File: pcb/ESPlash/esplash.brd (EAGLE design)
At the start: 100 x 70 mm, 55 parts, among them IC1 ACS712, K1 SRD-05VDC-SL-C, K2 SRD-05VDC-SL-C, K3 SRD-05VDC-SL-C, K4 SRD-05VDC-SL-C, Q1 SMD-TRANSISTORS-PNP-25V-500MA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, Q2 SMD-TRANSISTORS-PNP-25V-500MA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, Q3 SMD-TRANSISTORS-PNP-25V-500MA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, Q4 SMD-TRANSISTORS-PNP-25V-500MA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, U1 ESP-WROOM-32, U2 EL817(S)(D)(TU)-V, U3 EL817(S)(D)(TU)-V, U4 EL817(S)(D)(TU)-V, U5 EL817(S)(D)(TU)-V, Y1 ECS-.327-12.5-13X

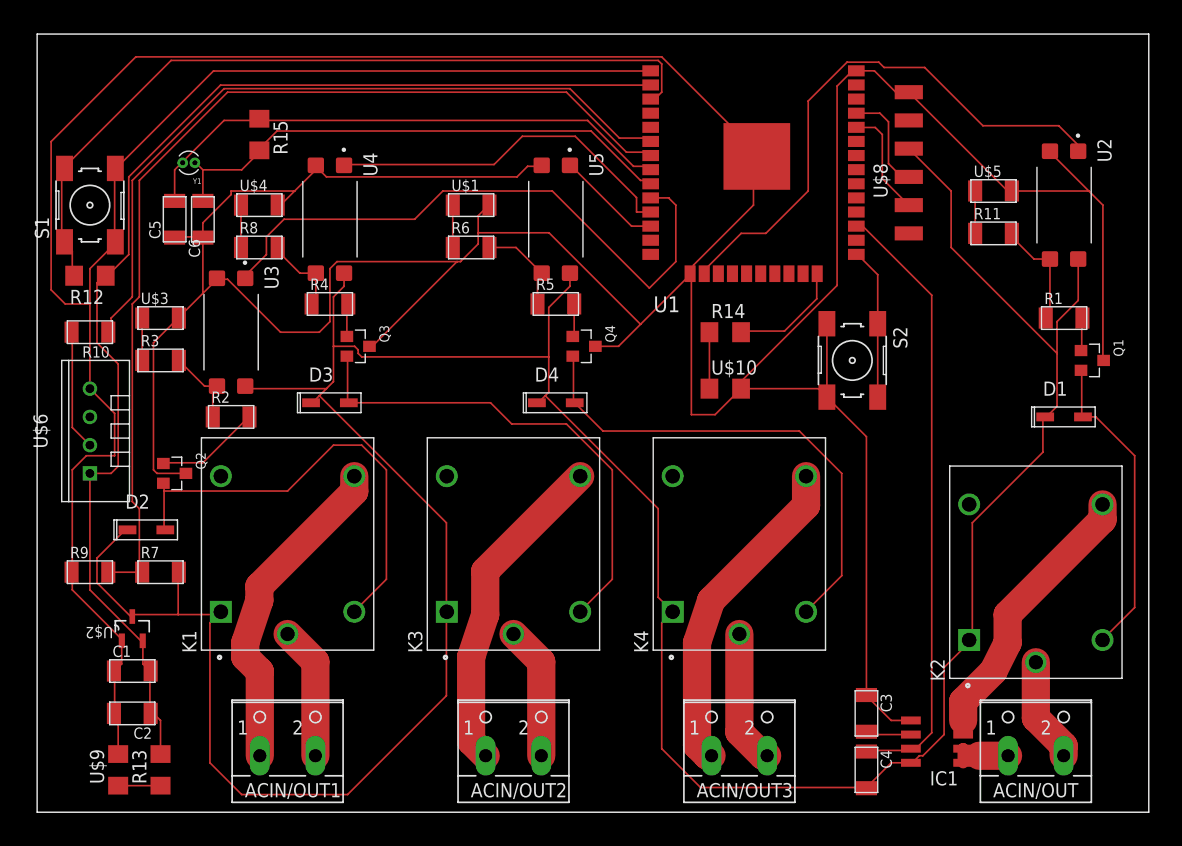
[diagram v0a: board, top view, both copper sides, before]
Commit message: pcb updates
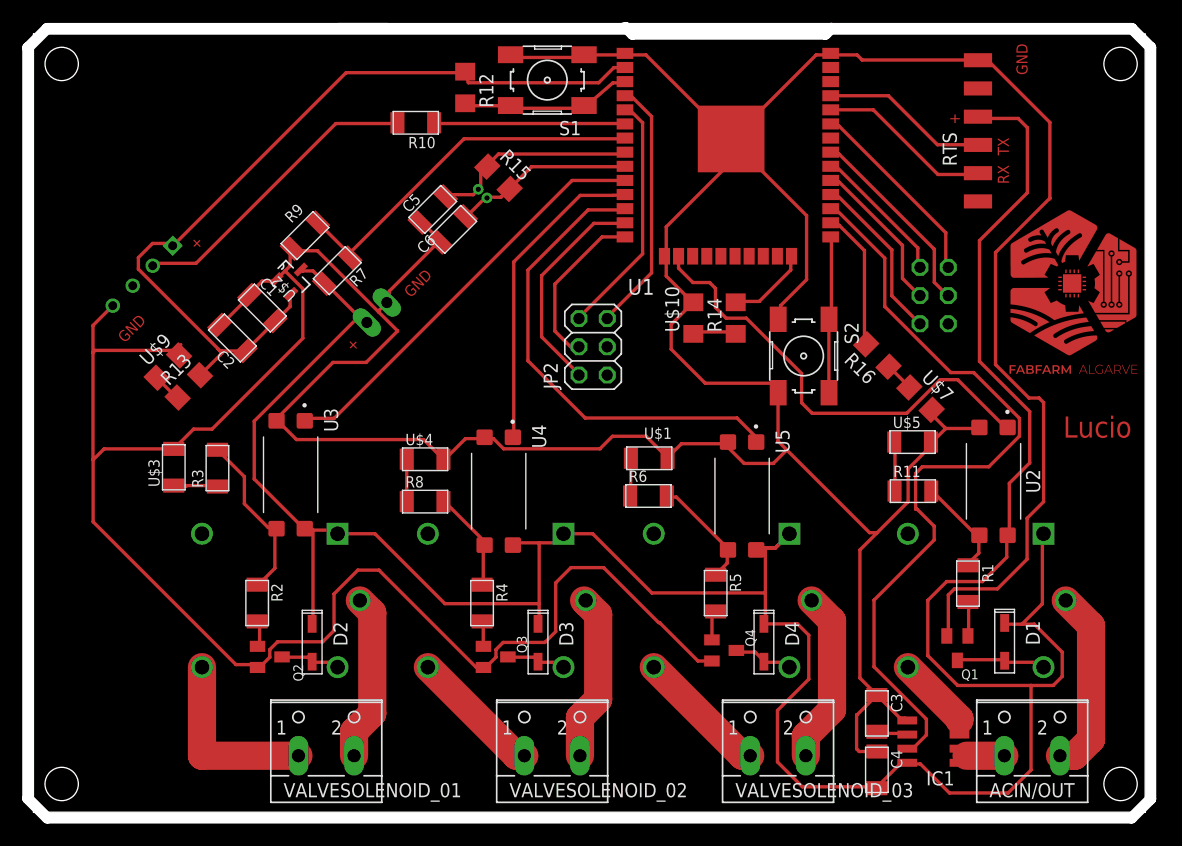
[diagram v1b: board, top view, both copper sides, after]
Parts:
- removed ACIN/OUT1, ACIN/OUT2, ACIN/OUT3: (no value), con-wago-500:W237-102
- removed U$8: FTDI-SMD-HEADER, fab:1X06SMD
- added JP1, JP2: header2x6, pinhead:2X03
- added POWER: 22-23-2021, con-molex:22-23-2021
- added R16: 100ohm, fab:R1206
- added RTS: FTDI-SMD-HEADER, fab:1X06SMD
- added U$7: LED, fab:LED1206
- added VALVESOLENOID_01, VALVESOLENOID_02, VALVESOLENOID_03: (no value), con-wago-500:W237-102
- C3: value (none) -> 1nF
- C4: value (none) -> 0.1uF
- C5, C6: value (none) -> 15pf
- Q1, Q2, Q3, Q4: value SMD-TRANSISTORS-PNP-25V-500MA(SOT-23) -> BCX70SMD; device SMD-TRANSISTORS-PNP-25V-500MA_SOT-23_:SOT-23 -> transistor:SOT23
- R10: value (none) -> 10K
- R11, R3, R6, R8: value (none) -> 100ohm
- R7: value (none) -> 1.2Mohm
- R9: value (none) -> 1.5Mohm
- S1: value (none) -> Reset
- S2: value (none) -> GPIO0 Button
- moved S1 42.7 mm to (46.2, 65.9), turned to 180 degrees
- moved R12 37.8 mm to (38.8, 65.2), turned to 270 degrees
- moved U$9 36.5 mm to (12.1, 40.1), turned to 45 degrees
- moved R9 35.9 mm to (24.4, 51.9), turned to 45 degrees
- moved C2 34.9 mm to (17.9, 42.7), turned to 135 degrees
- moved R10 34.8 mm to (34.4, 62.0)
- moved C1 34.7 mm to (20.6, 45.4), turned to 315 degrees
- moved U$2 34.7 mm to (23.3, 48.0), turned to 45 degrees
- moved R13 34.6 mm to (14.0, 38.3), turned to 45 degrees
- moved R7 31.4 mm to (27.3, 48.7), turned to 225 degrees
- moved Q3 30.6 mm to (41.6, 14.0)
- moved R4 30.2 mm to (40.4, 18.8), turned to 270 degrees
- moved Q4 30.1 mm to (62.1, 14.6)
- moved U5 30.0 mm to (63.7, 28.4)
- moved R5 29.7 mm to (61.4, 19.7), turned to 270 degrees
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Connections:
- net 3.3V renamed 3V3
- net AMP_M/IN renamed AMP_METER/IN
- net AMP_M/OUT renamed AMP_METER/OUT
- net GPIO1/PROGRAMER renamed GPIO0
- net N$41 renamed ACIN
- net RESET renamed CHIP_PU
- removed net 5V: C4.2, D1.CATHODE, D2.CATHODE, D3.CATHODE, D4.CATHODE, IC1.8, K1.A1, K2.A1, K3.A1, K4.A1, R7.2, U$2.3, U$8.3, U2.4, U3.4, U4.4, U5.4
- new net N$27: JP2.1
- new net N$28: JP2.3
- new net N$29: R16.1, U$7.1
- new net RTS: RTS.6
- new net VCC: C4.2, D1.CATHODE, D2.CATHODE, D3.CATHODE, D4.CATHODE, IC1.8, K1.A1, K2.A1, K3.A1, K4.A1, POWER.1, R7.2, RTS.3, U$2.3, U2.4, U3.4, U4.4, U5.4
- net GND: now also C4.1, POWER.2, Q1.2, Q2.2, Q3.2, Q4.2, RTS.1, U$7.2; no longer Q1.3, Q2.3, Q3.3, Q4.3, U$8.1
- net GPIO05: now also JP1.4
- net GPIO1/TXD0: now also RTS.4; no longer U$8.4
- net GPIO12: now also JP2.4
- net GPIO14: now also JP2.2
- net GPIO16/CURRENT_SENSE: no longer C4.1
- net GPIO17: now also JP1.6
- net GPIO18: now also JP1.2
- net GPIO19: now also JP1.3
- net GPIO21: now also JP1.1
- net GPIO3/RXD0: now also RTS.5; no longer U$8.5
- net GPIO36: now also JP2.5
- net GPIO39: now also JP2.6
- net GPIO4: now also R16.2
- net N$12: now also VALVESOLENOID_01.1; no longer ACIN/OUT1.1
- net N$15: now also VALVESOLENOID_02.2; no longer ACIN/OUT2.2
- net N$19: now also VALVESOLENOID_02.1; no longer ACIN/OUT2.1
- net N$20: now also VALVESOLENOID_03.2; no longer ACIN/OUT3.2
- net N$24: now also VALVESOLENOID_03.1; no longer ACIN/OUT3.1
- net N$5: now also VALVESOLENOID_01.2; no longer ACIN/OUT1.2
- net PUMPRELAYSEGMENT: now also Q1.3; no longer Q1.2
- net RELAY1SEGMENT: now also Q2.3; no longer Q2.2
- net RELAY2SEGMENT: now also Q3.3; no longer Q3.2
- net RELAY3SEGMENT: now also Q4.3; no longer Q4.2
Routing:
- net 5V: track 285.9 -> 0.00 mm
- net VCC: track 0.00 -> 256.4 mm
- net GPIO35/BATTVOLT: track 90.5 -> 33.8 mm
- net CHIP_PU: track 72.3 -> 16.6 mm
- net GPIO34/DHT: track 66.7 -> 17.2 mm
- net RELAY3SEGMENT: track 44.8 -> 5.47 mm
- net RELAY2SEGMENT: track 44.5 -> 5.41 mm
- net RELAY1SEGMENT: track 40.9 -> 5.40 mm
- net 3V3: track 109.7 -> 76.1 mm
- net GPIO27/VALVE_RELAY03: track 9.58 -> 43.0 mm
- net 32K_XN: track 47.7 -> 16.2 mm
- net 32K_XP: track 49.6 -> 18.6 mm
- net GPIO36: track 0.00 -> 23.1 mm
- net GND: track 501.9 -> 479.8 mm
- net GPIO39: track 0.00 -> 22.1 mm
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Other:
- board size 100 x 70 mm -> 101 x 71.1 mm
- board text added: "+"
- board text added: "GND"
- board text added: "Lucio"
- board text added: "RX"
- board text added: "TX"
